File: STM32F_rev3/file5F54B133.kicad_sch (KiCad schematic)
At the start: 43 parts, among them U10 SensorsV1, U11 SensorsV1, U12 SensorsV1, U13 SensorsV1, U14 SensorsV1, U15 SensorsV1, U16 SensorsV1, U17 SensorsV1, U18 SensorsV1, U19 SensorsV1, U2 SensorsV1, U27 LM321, U31 LM321, U32 LM321, U8 SensorsV1, U9 SensorsV1

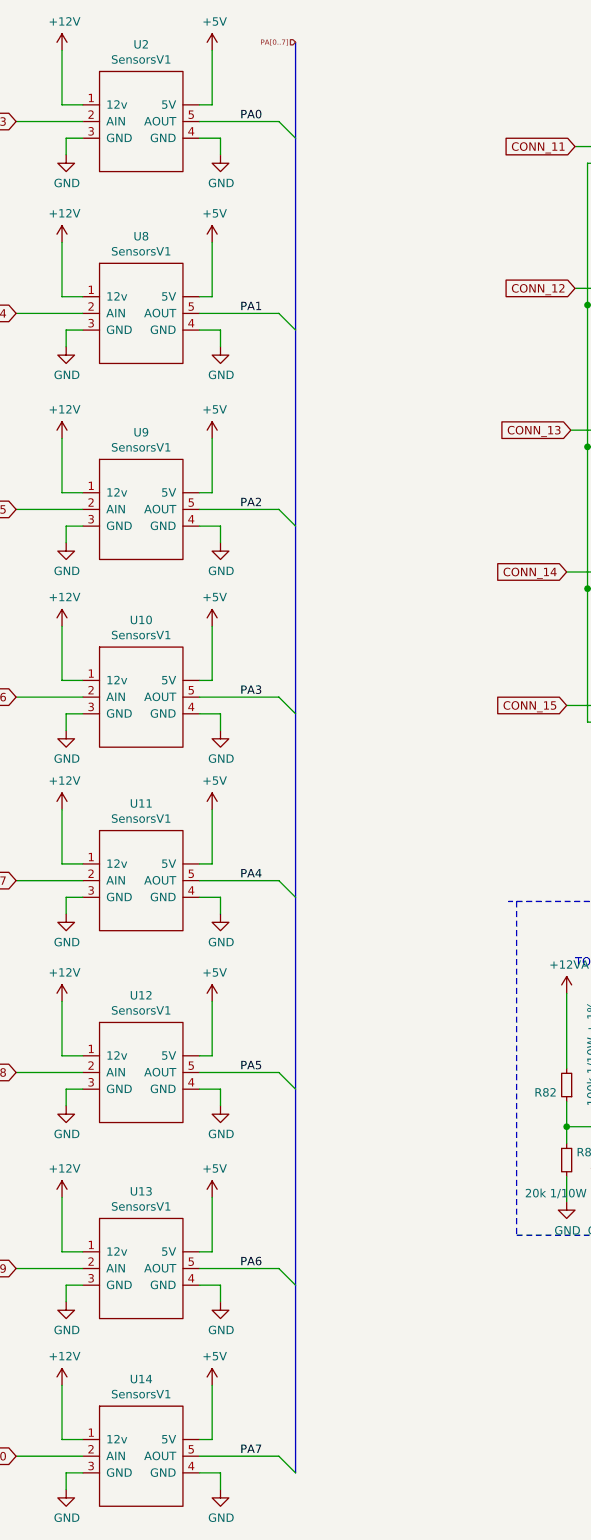
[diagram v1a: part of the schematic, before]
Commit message: Last commit to rev3
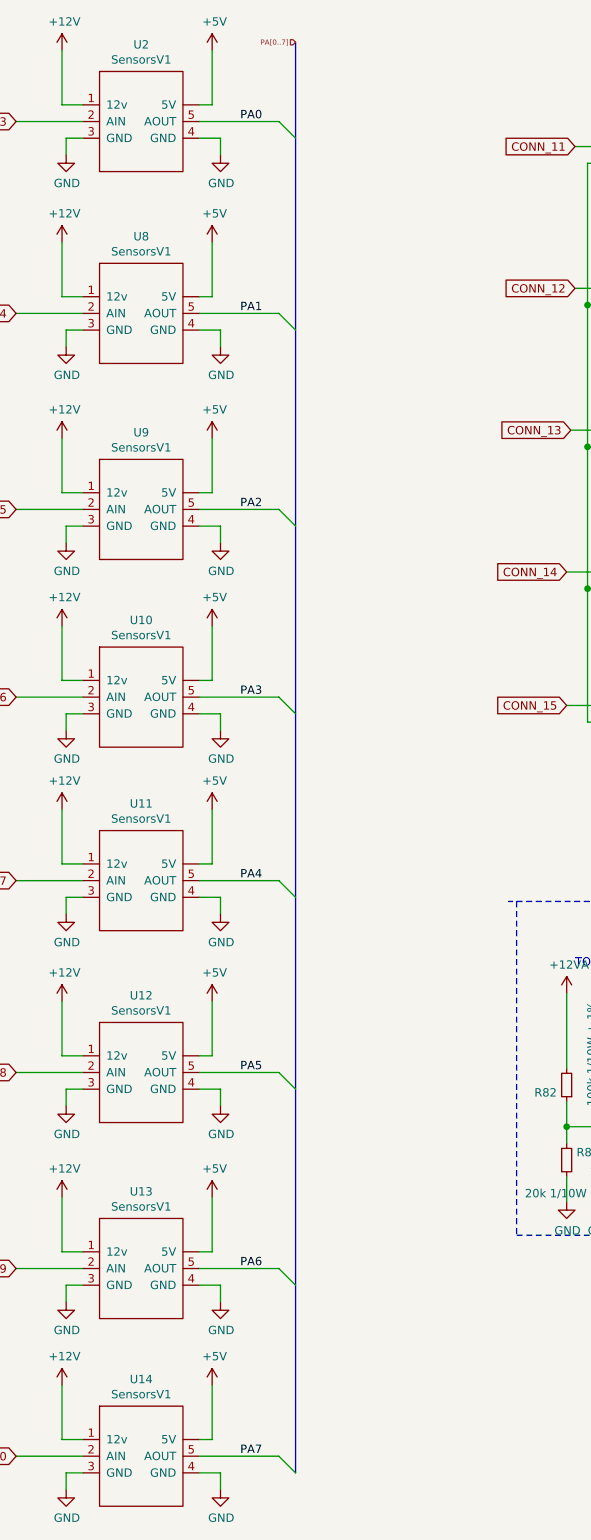
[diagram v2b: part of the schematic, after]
